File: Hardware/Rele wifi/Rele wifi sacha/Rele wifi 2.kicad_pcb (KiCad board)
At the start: 2 copper layers, 70 x 50 mm, 16 parts, among them J1 Screw_Terminal_01x02, J2 Screw_Terminal_01x03, J4 Conn_01x03_Pin, K1 G5LE-1, Q2 BC337, SW1 SW_Push, U5 PC817

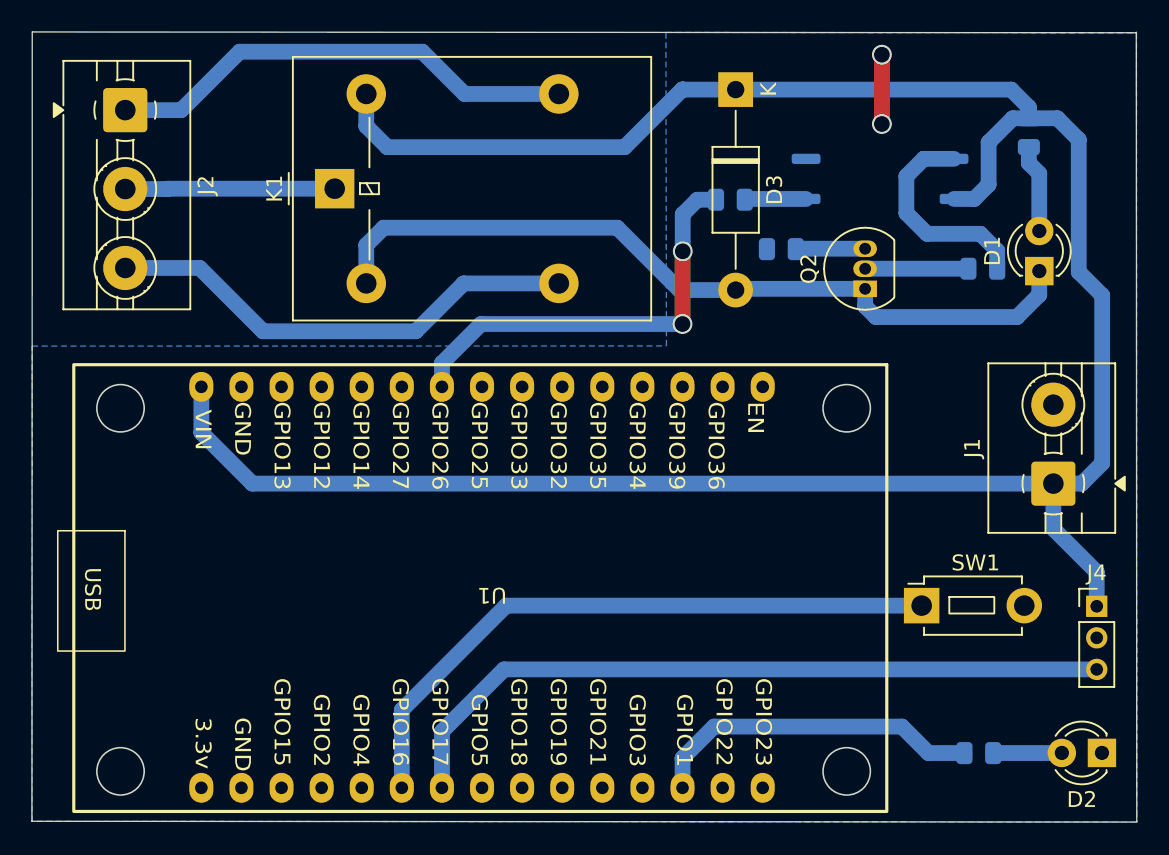
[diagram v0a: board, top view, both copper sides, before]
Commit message: actu pcb
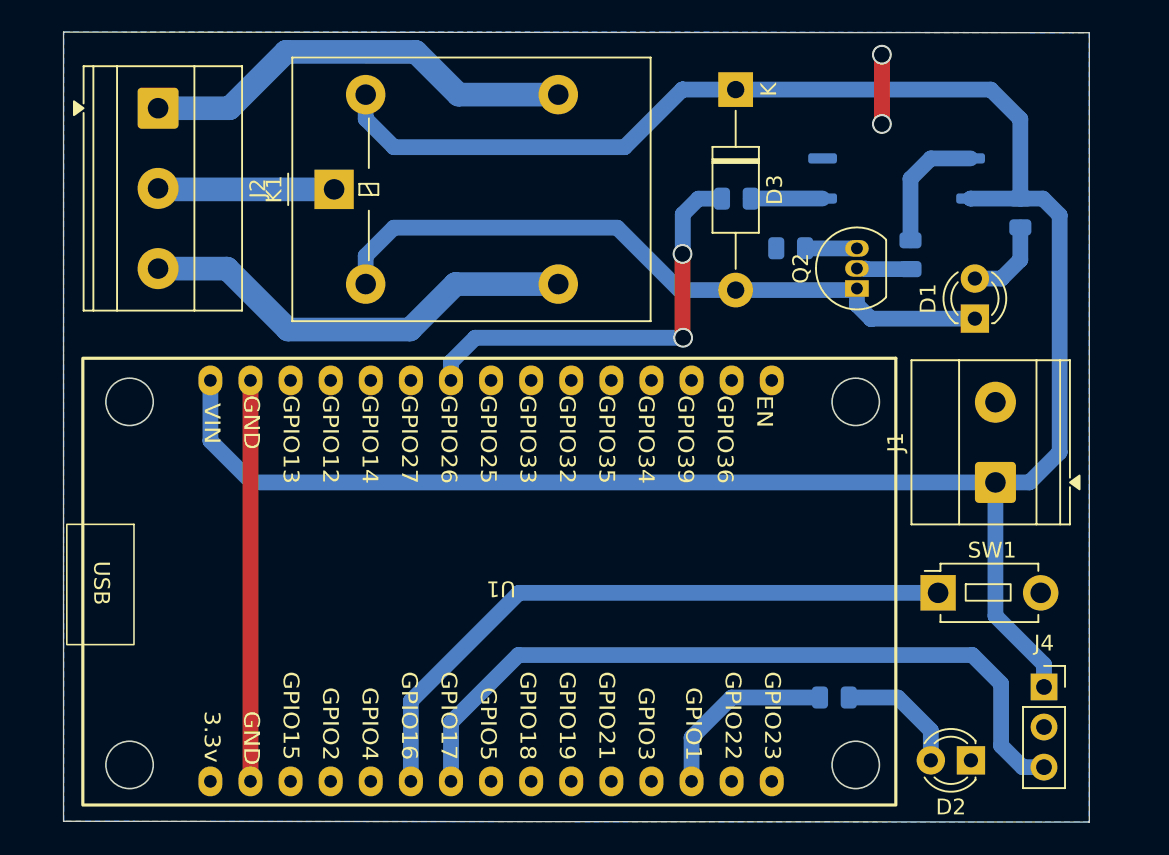
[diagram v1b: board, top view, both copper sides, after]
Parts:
- J1: footprint TerminalBlock:TerminalBlock_MaiXu_MX126-5.0-02P_1x02_P5.00mm -> TerminalBlock_Phoenix:TerminalBlock_Phoenix_MKDS-1,5-2-5.08_1x02_P5.08mm_Horizontal
- J2: footprint TerminalBlock:TerminalBlock_MaiXu_MX126-5.0-03P_1x03_P5.00mm -> TerminalBlock_Phoenix:TerminalBlock_Phoenix_MKDS-1,5-3-5.08_1x03_P5.08mm_Horizontal
- J4: footprint Connector_PinHeader_2.00mm:PinHeader_1x03_P2.00mm_Vertical -> Connector_PinSocket_2.54mm:PinSocket_1x03_P2.54mm_Vertical
- moved R5 9.80 mm to (201.2, 79.1)
- moved D2 8.31 mm to (209.8, 83.1)
- moved J4 6.10 mm to (214.4, 78.4)
- moved R1 5.12 mm to (212.9, 48.4)
- moved D1 5.07 mm to (210.1, 55.1)
- moved R2 4.67 mm to (206.0, 51.1), turned to -90 degrees
- moved J1 3.67 mm to (211.4, 65.5)
- moved J2 2.08 mm to (158.3, 41.8)
- moved SW1 1.32 mm to (207.7, 72.5)
- moved U5 1.05 mm to (205.1, 46.2)
- moved U1 0.70 mm to (178.7, 71.0)
- moved R4 0.59 mm to (198.4, 50.6)
- moved Q2 0.52 mm to (202.6, 53.2)
- moved R3 0.38 mm to (195.0, 47.5)
- moved K1 0.06 mm to (169.5, 46.9)
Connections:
- net VIN renamed +5V
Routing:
- net GND: track 4.39 -> 29.8 mm
- net GPIO4: track 21.3 -> 12.0 mm
- net Net-(D1-K): track 50.7 -> 43.8 mm
- net Net-(R2-Pad1): track 13.7 -> 8.24 mm
- net +5V: track 151.3 -> 146.0 mm
- net Net-(Q2-B): track 6.56 -> 2.89 mm
- net Net-(D2-A): track 4.35 -> 7.95 mm
- net NC: track 30.4 -> 28.1 mm
- net NO: track 30.1 -> 27.9 mm
- net COM: track 13.3 -> 11.3 mm
- net GPIO14: track 46.7 -> 48.3 mm
- net GPIO12: track 40.6 -> 41.7 mm
- net Net-(Q2-E): track 4.41 -> 3.29 mm
- net Net-(R3-Pad2): track 3.90 -> 4.55 mm
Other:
- board size 70 x 50 mm -> 65 x 50 mm
